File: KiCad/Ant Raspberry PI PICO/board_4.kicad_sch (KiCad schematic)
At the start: 13 parts

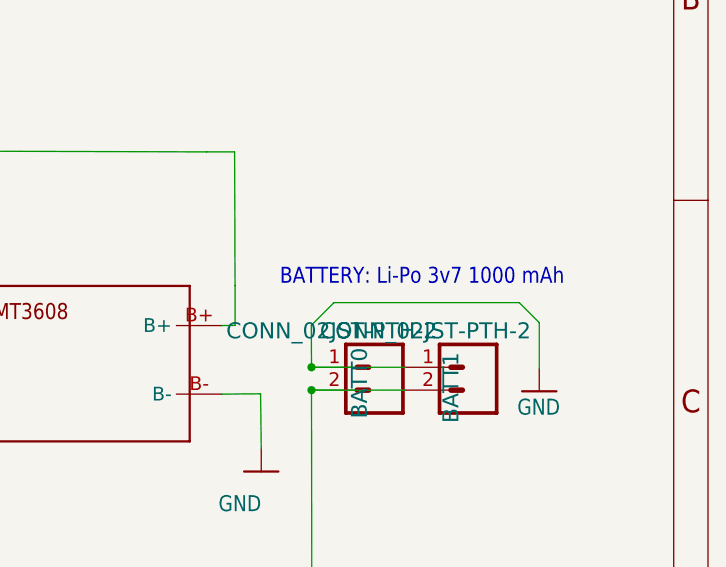
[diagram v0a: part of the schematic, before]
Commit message: Mensaje describiendo tus cambios
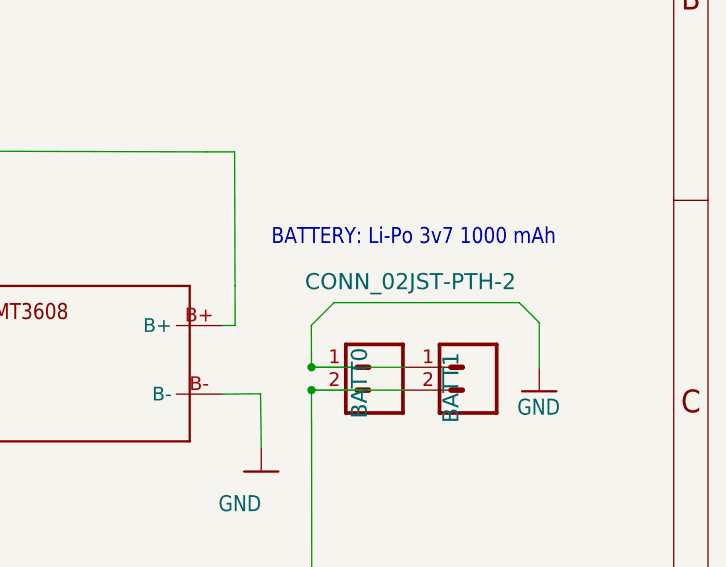
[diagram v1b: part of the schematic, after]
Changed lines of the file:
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@@
 	(text "BATTERY: Li-Po 3v7 1000 mAh"
 		(exclude_from_sim no)
-		(at 231.826 97.894 0)
+		(at 230.886 93.472 0)
 		(effects
 			(font
@@
 		)
 		(property "Value" "CONN_02JST-PTH-2"
-			(at 249.3146 101.7318 0)
+			(at 258.064 96.266 0)
 			(effects
 				(font
@@
 				)
 				(justify left bottom)
-			)
-		)
+				(hide yes)
+			)
+		)
